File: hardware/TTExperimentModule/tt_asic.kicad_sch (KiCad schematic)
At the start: 22 parts, among them J5 Conn_01x04, U4 Openframe_QFN_TT06_REV2

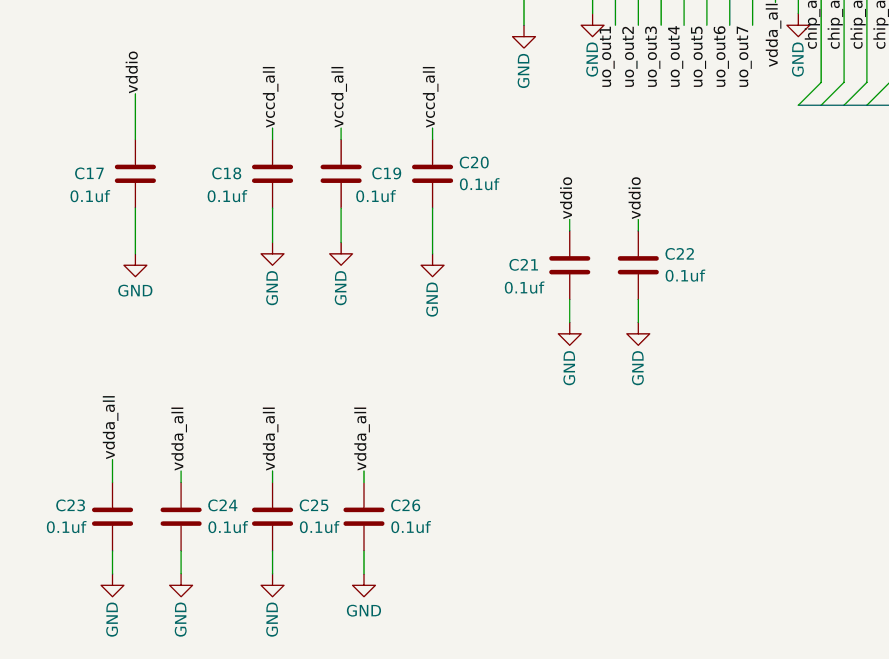
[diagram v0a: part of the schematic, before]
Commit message: BOM updates for spaaaaaace
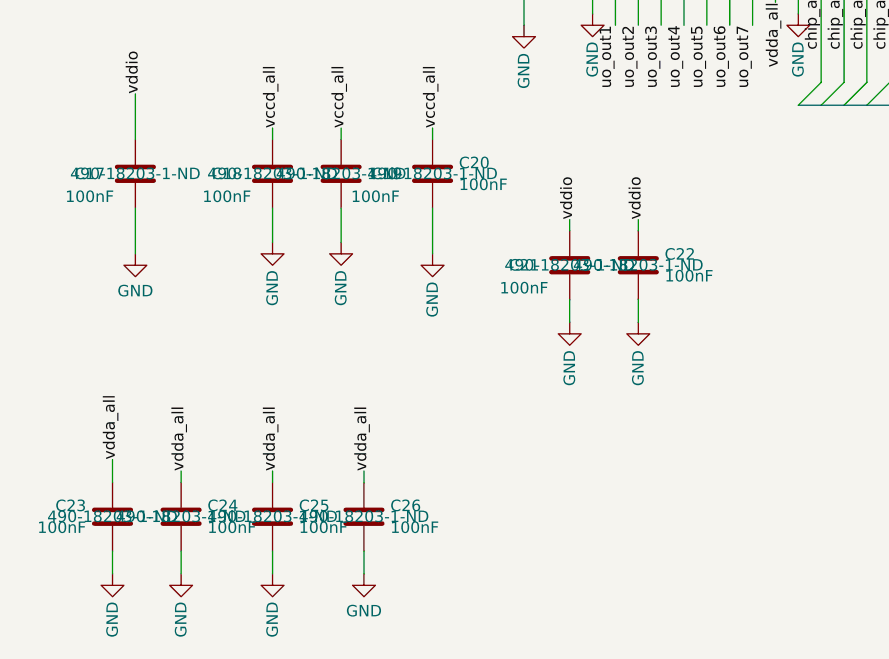
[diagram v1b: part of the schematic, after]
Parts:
- C12, C14, C15, C16, C8: value C_1u_0603_50V -> 1uF; DigikeyPN 490-12330-1-ND -> 587-3410-1-ND; LCSC C5673 -> (none); MPN GRT188R61H105KE13D -> LMK107B7105KAHT
- C17, C18, C19, C20, C21, C22, C23, C24, C25, C26: value 0.1uf -> 100nF; DigikeyPN (none) -> 490-18203-1-ND; LCSC C100072 -> (none); MPN CL05A104KA5NNNC -> GCM155L81E104KE02D
- R11: DigikeyPN (none) -> 10-ERJ-H2GJ102XCT-ND; LCSC C202394 -> (none); MPN (none) -> ERJ-H2GJ102X
- R7, R8: DigikeyPN (none) -> 738-RMCF1206ZG0R00CT-ND; MPN (none) -> RMCF1206ZG0R00
- R9: LCSC C202394 -> (none)
